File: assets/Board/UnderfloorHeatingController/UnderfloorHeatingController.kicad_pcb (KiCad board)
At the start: 2 copper layers, 172.7 x 52.3 mm, 54 parts, among them J10 Screw_Terminal_01x02, J11 Screw_Terminal_01x02, J12 Screw_Terminal_01x02, J13 Screw_Terminal_01x02, J14 Screw_Terminal_01x02, J15 Screw_Terminal_01x02, J16 Screw_Terminal_01x02, J2 Screw_Terminal_01x03, J3 Screw_Terminal_01x03, J5 Screw_Terminal_01x02, J6 Screw_Terminal_01x02, J7 Screw_Terminal_01x02, J8 Screw_Terminal_01x02, J9 Screw_Terminal_01x02, K1 G5Q-1A, Q1 BC337, U10 AQY214EH, U11 AQY214EH, U12 AQY214EH, U13 AQY214EH, U14 AQY214EH, U15 AQY214EH, U16 AQY214EH, U2 Waveshare_ESP32-S3-Tiny, U4 AQY214EH, U5 ACS725LLCTR-10AB-T, U6 AQY214EH, U7 AQY214EH, U8 AQY214EH, U9 AQY214EH

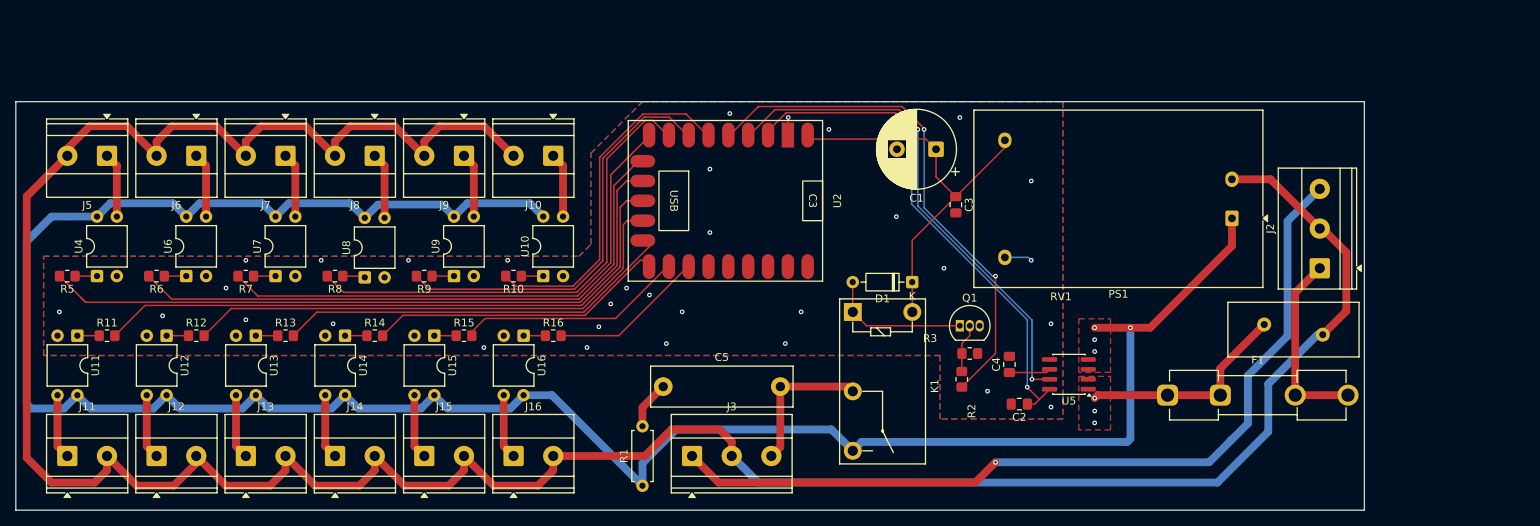
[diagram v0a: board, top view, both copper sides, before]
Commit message: Minor tweaks.
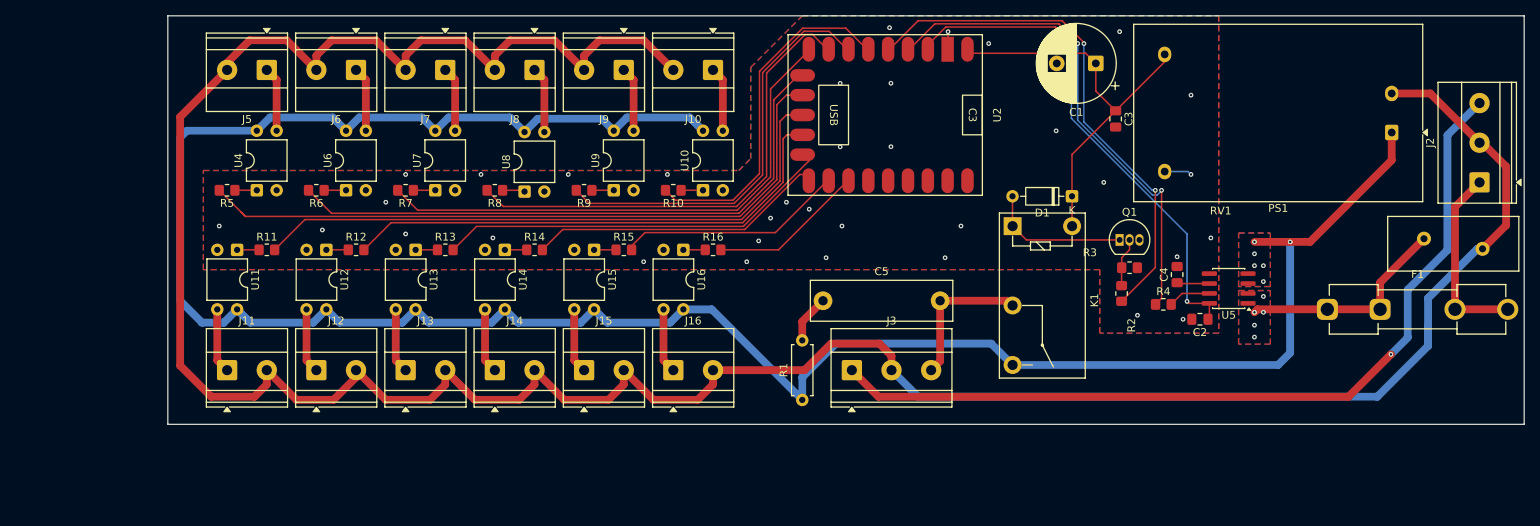
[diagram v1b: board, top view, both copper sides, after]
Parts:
- added R4: 100, Resistor_SMD:R_0805_2012Metric_Pad1.20x1.40mm_HandSolder, F.Cu at (173.4, 102.7)
- moved C2 25.6 mm to (178.1, 104.6)
- moved C4 24.4 mm to (175.2, 98.9)
- moved R15 23.2 mm to (104.3, 95.7)
- moved C5 23.2 mm to (129.8, 102.2)
- moved J8 23.2 mm to (92.8, 72.6)
- moved R13 23.2 mm to (81.4, 95.7)
- moved U14 23.2 mm to (89.0, 95.7)
- moved U16 23.2 mm to (111.9, 95.7)
- moved J12 23.2 mm to (64.9, 111.1)
- moved J5 23.2 mm to (58.6, 72.6)
- moved J6 23.2 mm to (70.0, 72.6)
- moved R5 23.2 mm to (53.5, 88.1)
- moved R7 23.2 mm to (76.3, 88.1)
- moved U12 23.2 mm to (66.2, 95.7)
- moved U4 23.2 mm to (57.3, 88.1)
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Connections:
- U5 pad 7: CURRENT_MON -> Net-(U5-VIOUT)
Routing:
- net Net-(U5-VIOUT): track 0.00 -> 5.47 mm
- net POWER_N: track 356.0 -> 359.2 mm
- net POWER_L_MON: track 295.6 -> 297.3 mm, vias 4 -> 6
- net Net-(U5-FILTER): track 5.31 -> 4.17 mm
- net +3V3: track 66.6 -> 65.8 mm
- net CURRENT_MON: track 67.3 -> 66.7 mm
- net GND: vias 33 -> 36
- net POWER_L: vias 3 -> 5
- added copper zone on B.Cu, net POWER_L
- added copper zone on B.Cu, net POWER_L_MON
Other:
- board size 172.7 x 52.3 mm -> 173.7 x 52.3 mm
